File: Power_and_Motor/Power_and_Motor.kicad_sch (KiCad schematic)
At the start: 21 parts, among them M1 Motor_DC, Q1 BC337, Q2 BC337, SW1 SW_DPDT_x2, U1 LM317_TO-220

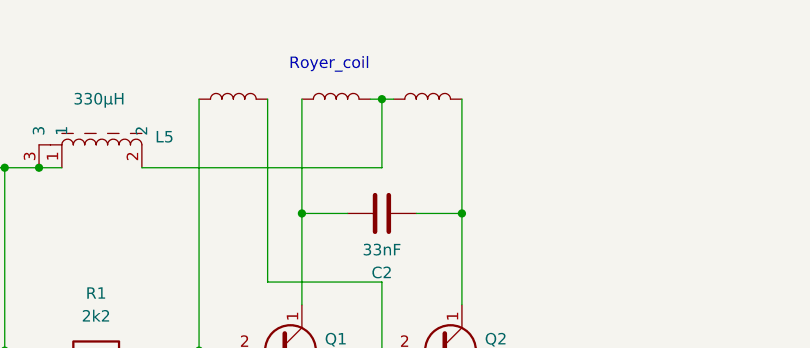
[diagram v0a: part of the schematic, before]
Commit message: AddComponant
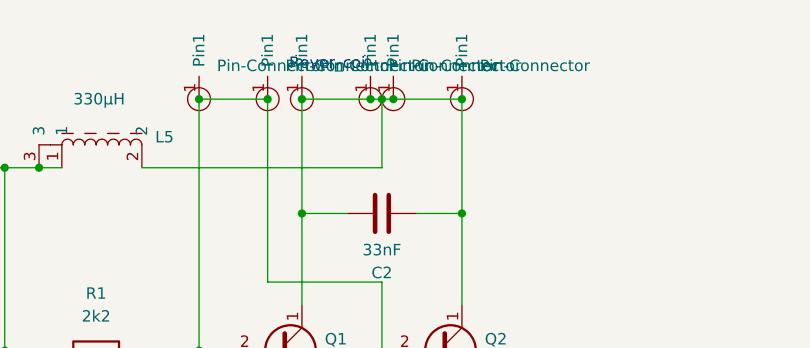
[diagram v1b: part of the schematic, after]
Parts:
- removed L2, L3, L4: L, symbol Device:L
- added U2, U3, U4, U5, U6, U7: Pin-Connector, my_footprints:Pin_2mm, symbol my_symbols:Pin-Connector
- Q1: footprint Package_TO_SOT_THT:TO-92_Inline -> Package_TO_SOT_THT:TO-92_Inline_Wide
- Q2: footprint Package_TO_SOT_THT:TO-92_Inline -> Package_TO_SOT_THT:TO-92L_Inline_Wide
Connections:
- net at C2.1, Q1.1 (C): now also C2.2, L5.2, Q2.1 (C), U4.1 (Pin1), U5.1 (Pin1), U6.1 (Pin1), U7.1 (Pin1)
- net at Q1.2 (B), R1.2: now also Q2.2 (B), U2.1 (Pin1), U3.1 (Pin1)
